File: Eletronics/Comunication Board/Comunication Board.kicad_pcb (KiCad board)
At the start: 2 copper layers, 39.5 x 40.1 mm, 36 parts, among them J1 USB_C_Receptacle_USB2.0, J2 Conn_01x10_Female, T1 AMS1117/3V3, U1 BATERIA, U2 ESP32-S3-WROOM-1-N8R2

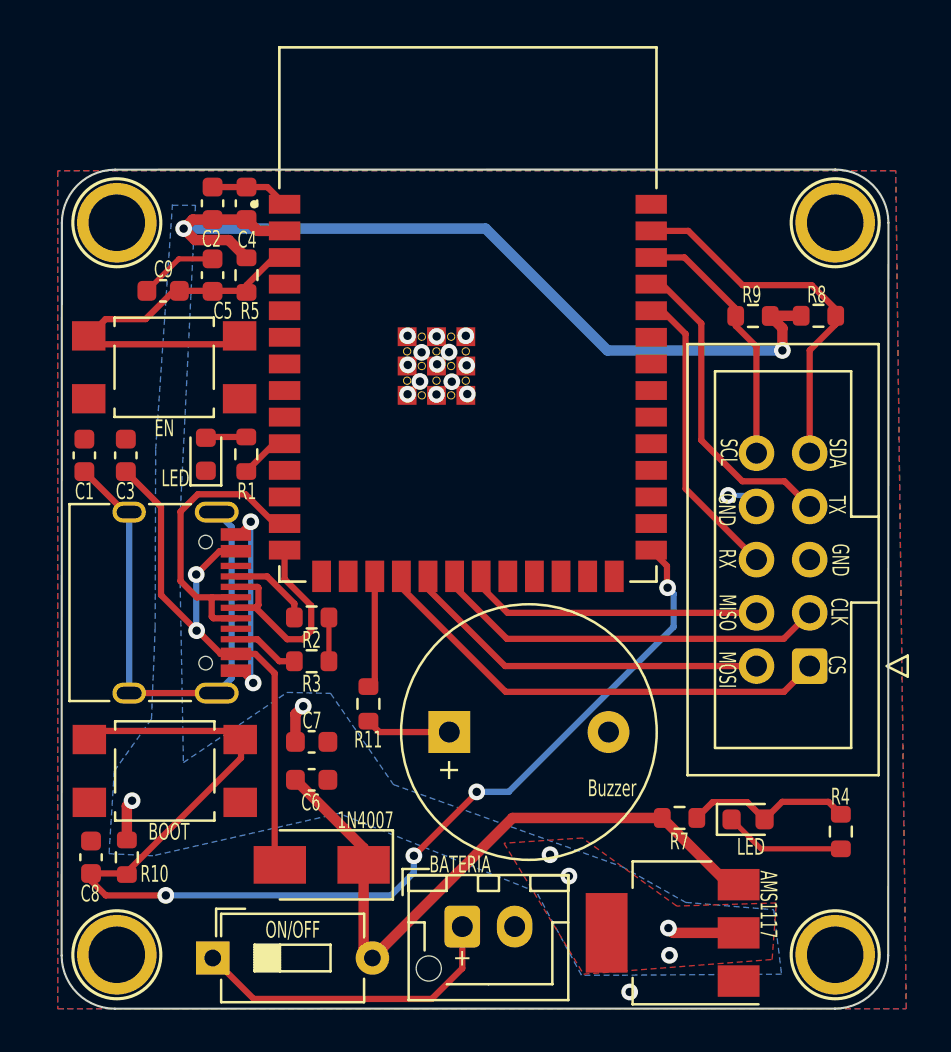
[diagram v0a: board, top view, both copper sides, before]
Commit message: Atualização do repositório
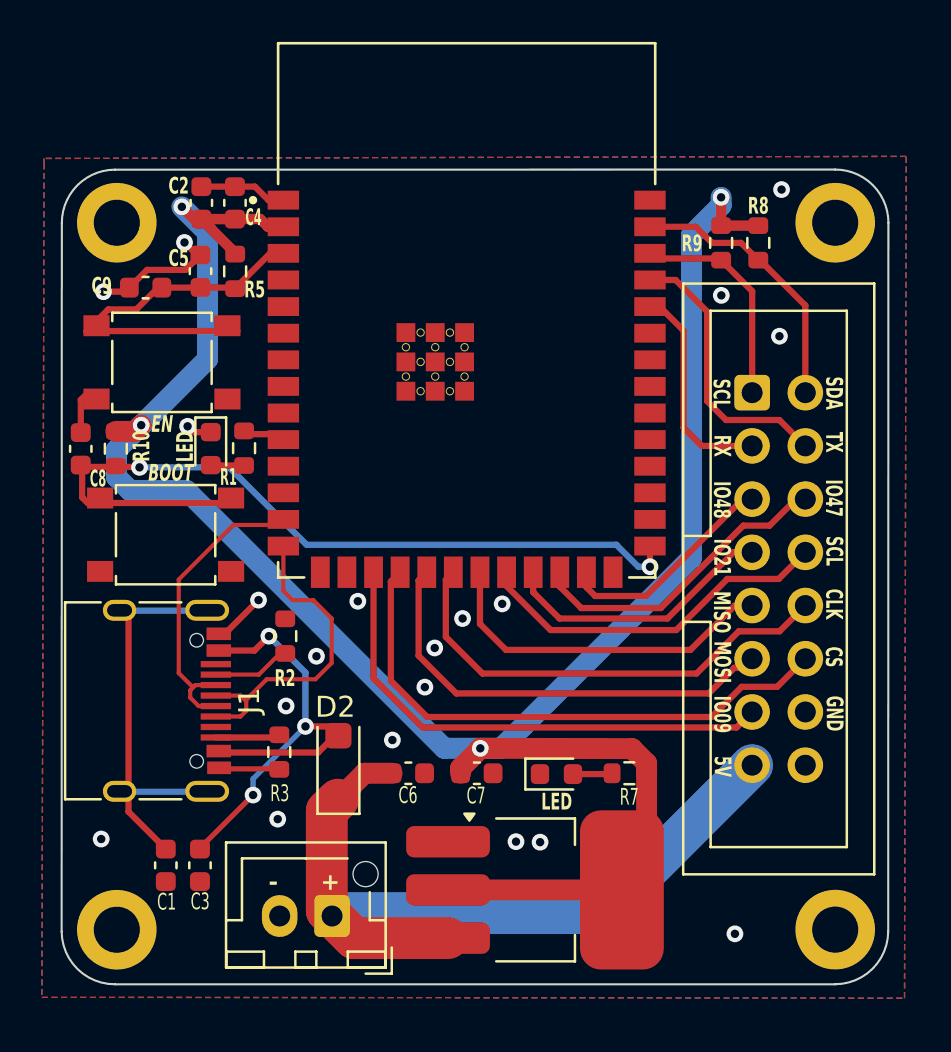
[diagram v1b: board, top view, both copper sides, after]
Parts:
- removed BOOT1: SW_Push, Button_Switch_SMD:SW_SPST_TL3305A
- removed BZ1: Buzzer, Buzzer_Beeper:Buzzer_12x9.5RM7.6
- removed D1: 1N4007, Diode_SMD:D_SMA
- removed the EN1 at (132.6, 74.9)
- removed H1, H2, H3, H4: MountingHole, SirBoardLibrary:MountingHole_M2.5_SirBoard
- removed POWER1: ON/OFF, Button_Switch_THT:SW_DIP_SPSTx01_Slide_6.7x4.1mm_W7.62mm_P2.54mm_LowProfile
- removed R11: 330 Ω, Resistor_SMD:R_0603_1608Metric
- removed R4: 1.5 KΩ, Resistor_SMD:R_0603_1608Metric
- added 1: MountingHole_2.2mm_M2_DIN965_Pad, MountingHole:MountingHole_2.2mm_M2_DIN965_Pad, F.Cu at (130.3, 101.7)
- added 2: MountingHole_2.2mm_M2_DIN965_Pad, MountingHole:MountingHole_2.2mm_M2_DIN965_Pad, F.Cu at (130.3, 68.0)
- added 3: MountingHole_2.2mm_M2_DIN965_Pad, MountingHole:MountingHole_2.2mm_M2_DIN965_Pad, F.Cu at (164.6, 68.0)
- added 4: MountingHole_2.2mm_M2_DIN965_Pad, MountingHole:MountingHole_2.2mm_M2_DIN965_Pad, F.Cu at (164.6, 101.7)
- added D2: SS34, Diode_SMD:D_SOD-123F, F.Cu at (140.9, 93.7)
- added EN1: SW_Push, Button_Switch_SMD:SW_SPST_TL3305A, F.Cu at (132.7, 82.9)
- added EN1: SW_Push, Button_Switch_SMD:SW_SPST_TL3305A, F.Cu at (132.5, 74.7)
- C7: value 10 uF -> 22 uF
- J1: footprint c:USB_C_Receptacle_HRO_TYPE-C-31-M-12 -> usb_type_C:USB_C_Receptacle_KH-TYPE-C-16P
- J2: value Conn_01x10_Female -> Conn_01x16_Socket; footprint Connector_IDC:IDC-Header_2x05_P2.54mm_Vertical -> Connector_IDC:IDC-Header_2x08_P2.54mm_Vertical
- R7: value 330 Ω -> 130 Ω
- U1: value BATERIA -> VCC
- U2: footprint lib:XCVR_ESP32-S3-WROOM-1-N8R2 -> ESP32-S3-WROOM-1-N8R2:XCVR_ESP32-S3-WROOM-1-N8R2
- moved C1 20.0 mm to (132.7, 98.7), turned to -90 degrees
- moved C3 19.9 mm to (134.3, 98.7), turned to -90 degrees
- moved R10 19.5 mm to (130.3, 78.8)
- moved C8 19.5 mm to (128.6, 78.8)
- moved J2 13.3 mm to (160.6, 76.1), turned to 0 degrees
- moved L4 9.40 mm to (151.3, 94.3)
- moved C7 8.03 mm to (147.5, 94.3)
- moved T1 6.88 mm to (150.3, 99.8), turned to 0 degrees
- moved U1 6.24 mm to (140.6, 101.1), turned to 180 degrees
- moved J1 4.79 mm to (131.0, 90.8)
- moved C6 4.62 mm to (144.2, 94.3)
- moved R3 4.60 mm to (138.1, 93.2), turned to -90 degrees
- moved R8 4.51 mm to (160.9, 68.9), turned to -90 degrees
- moved R9 3.81 mm to (159.2, 68.9), turned to -90 degrees
- moved R7 3.21 mm to (154.8, 94.3), turned to 180 degrees
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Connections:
- J1 pad A6: USB_D- -> USB_D+
- J1 pad A7: USB_D+ -> USB_D-
- J1 pad B6: USB_D- -> USB_D+
- J1 pad B7: USB_D+ -> USB_D-
- J2 pad 1: SPI_CS -> SCL
- J2 pad 10: SCL -> SPI_CLK
- J2 pad 2: SPI_MOSI -> SDA
- J2 pad 3: SPI_CLK -> RXD0
- J2 pad 4: SPI_MISO -> TXD0
- J2 pad 5: GNDREF -> GPIO48
- J2 pad 6: RXD0 -> GPIO47
- J2 pad 7: TXD0 -> GPIO21
- J2 pad 8: GNDREF -> GPIO14
- J2 pad 9: SDA -> SPI_MISO
- R7 pad 1: +5V -> +3.3V
- U1 pad 1: Net-(POWER1-Pad1) -> +5V
- U2 pad 22: unconnected-(U2-Pad22) -> GPIO14
- U2 pad 23: unconnected-(U2-Pad23) -> GPIO21
- U2 pad 24: unconnected-(U2-Pad24) -> GPIO47
- U2 pad 25: unconnected-(U2-Pad25) -> GPIO48
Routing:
- net +3.3V: track 51.3 -> 106.9 mm, vias 8 -> 4
- net GPIO9: track 5.39 -> 24.4 mm
- net GPIO14: track 0.00 -> 17.3 mm
- net I00: track 56.2 -> 39.4 mm, vias 4 -> 2
- net Net-(POWER1-Pad1): track 15.3 -> 0.00 mm
- net GPIO47: track 0.00 -> 15.0 mm
- net GPIO21: track 0.00 -> 13.2 mm
- net GPIO48: track 0.00 -> 10.7 mm
- net GNDREF: track 27.4 -> 18.8 mm, vias 17 -> 20
- net +5V: track 31.6 -> 38.0 mm
- net Net-(L4-A): track 8.12 -> 1.88 mm
- net Net-(D2-A): track 28.6 -> 23.7 mm, vias 2 -> 3
- net SDA: track 17.7 -> 13.1 mm
- net Net-(J1-SHIELD): track 25.0 -> 20.5 mm
- net SPI_CS: track 22.6 -> 27.0 mm
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- removed copper zone on B.Cu, net +3.3V
- removed copper zone on F.Cu, net +3.3V
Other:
- board size 39.5 x 40.1 mm -> 39.5 x 38.9 mm
- board text added: "+"
- board text added: "-"
- board text added: "5V"
- board text added: "CLK"
- board text added: "CS"
- board text added: "GND"
- board text added: "IO09"
- board text added: "IO21"
- board text added: "IO47"
- board text added: "IO48"
- board text added: "LED"
- board text added: "MISO"
- board text added: "MOSI"
- board text added: "RX"
- board text added: "SCL"
- board text added: "SDA"
- board text added: "SSL Comms V1"
- board text added: "TX"
- board text removed: "SSL V1"
